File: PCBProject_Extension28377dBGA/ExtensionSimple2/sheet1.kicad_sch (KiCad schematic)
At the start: 88 parts, among them J1 Conn_02x05_Odd_Even, J1 Conn_02x08_Top_Bottom, J2 Conn_01x02_Pin, Q1 FMMT618TA, U1 SN74ABT541, U2 SN74ABT541

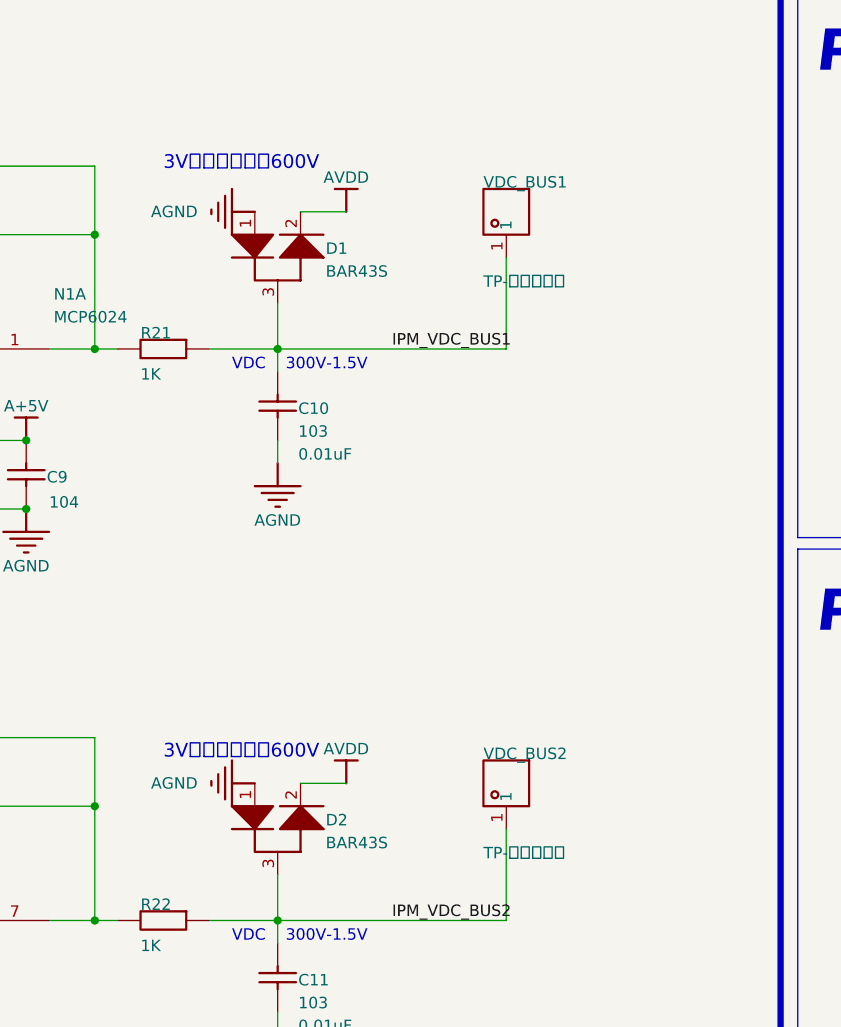
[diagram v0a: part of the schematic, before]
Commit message: corrret Extension size
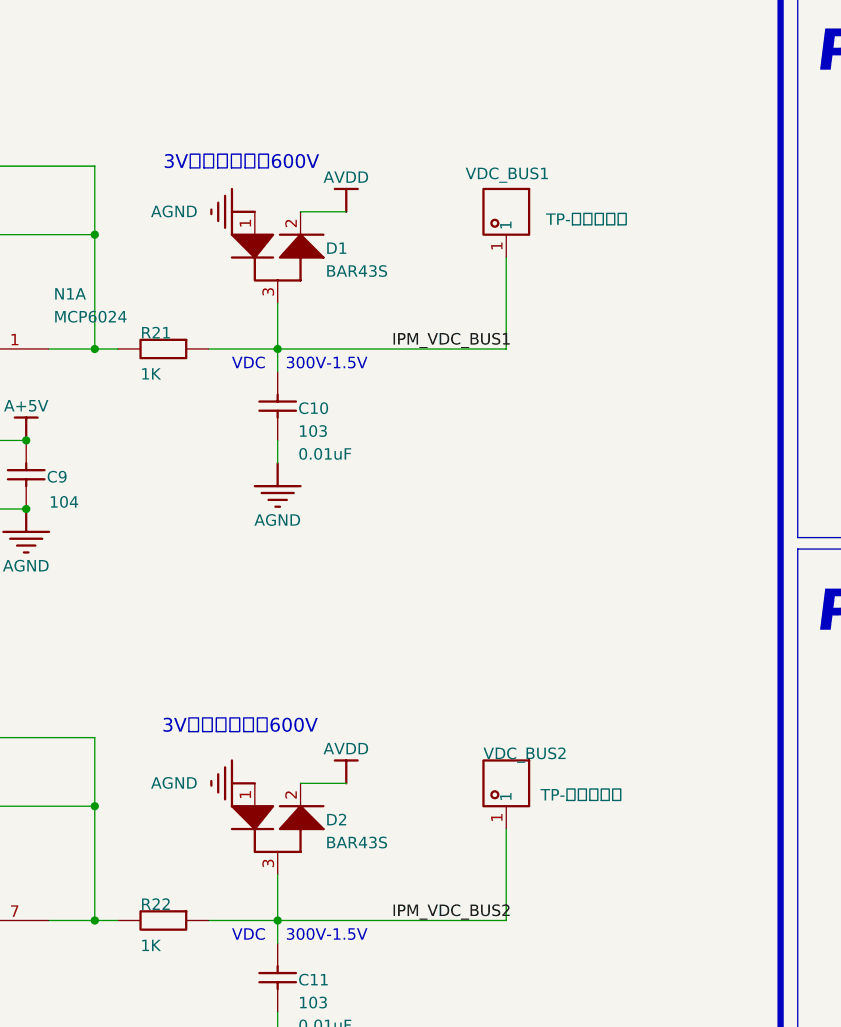
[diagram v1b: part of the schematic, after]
